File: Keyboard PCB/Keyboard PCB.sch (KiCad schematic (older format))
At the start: 15 parts

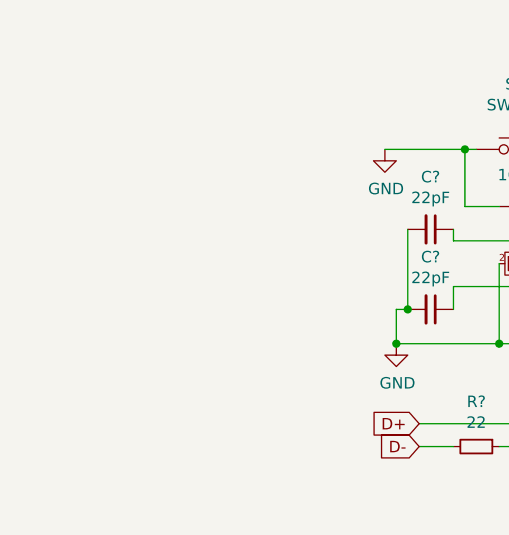
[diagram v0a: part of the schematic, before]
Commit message: Metidas las librerías acheron
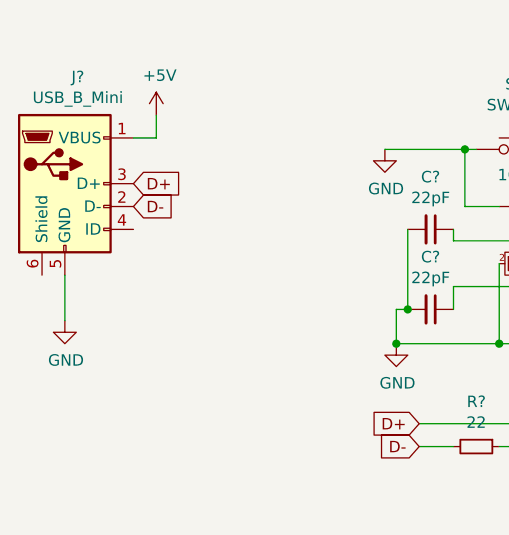
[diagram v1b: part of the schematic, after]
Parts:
- added J?: USB_B_Mini, symbol Connector:USB_B_Mini
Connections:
- wire segments 52 -> 55
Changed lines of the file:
@@
 EESchema Schematic File Version 4
+LIBS:Keyboard PCB-cache
 EELAYER 30 0
 EELAYER END
@@
 Wire Wire Line
 	5250 1050 4900 1050
+$Comp
+L Connector:USB_B_Mini J?
+U 1 1 5D835ABB
+P 3500 1200
+F 0 "J?" H 3557 1667 50  0000 C CNN
+F 1 "USB_B_Mini" H 3557 1576 50  0000 C CNN
+F 2 "" H 3650 1150 50  0001 C CNN
+F 3 "~" H 3650 1150 50  0001 C CNN
+	1    3500 1200
+	1    0    0    -1
+$EndComp
+$Comp
+L power:+5V #PWR?
+U 1 1 5D837687
+P 3900 900
+F 0 "#PWR?" H 3900 750 50  0001 C CNN
+F 1 "+5V" H 3915 1073 50  0000 C CNN
+F 2 "" H 3900 900 50  0001 C CNN
+F 3 "" H 3900 900 50  0001 C CNN
+	1    3900 900
+	1    0    0    -1
+$EndComp
+Text GLabel 3800 1200 2    50   Input ~ 0
+D+
+Text GLabel 3800 1300 2    50   Input ~ 0
+D-
+Wire Wire Line
+	3800 1000 3900 1000
+Wire Wire Line
+	3900 1000 3900 900
+$Comp
+L power:GND #PWR?
+U 1 1 5D83AD54
+P 3500 1800
+F 0 "#PWR?" H 3500 1550 50  0001 C CNN
+F 1 "GND" H 3505 1627 50  0000 C CNN
+F 2 "" H 3500 1800 50  0001 C CNN
+F 3 "" H 3500 1800 50  0001 C CNN
+	1    3500 1800
+	1    0    0    -1
+$EndComp
+Wire Wire Line
+	3500 1600 3500 1800
 $EndSCHEMATC
